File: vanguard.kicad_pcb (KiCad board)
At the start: 4 copper layers, 27.5 x 33.4 mm, 30 parts, among them J1 Conn_01x02, J2 USB_C_Receptacle, J3 Conn_01x04_Pin, J4 Conn_01x02, SW1 Switch_Tactile_CnK, U1 ATtiny3227-M, U2 MCP73831-2-OT, U5 AP63203WU

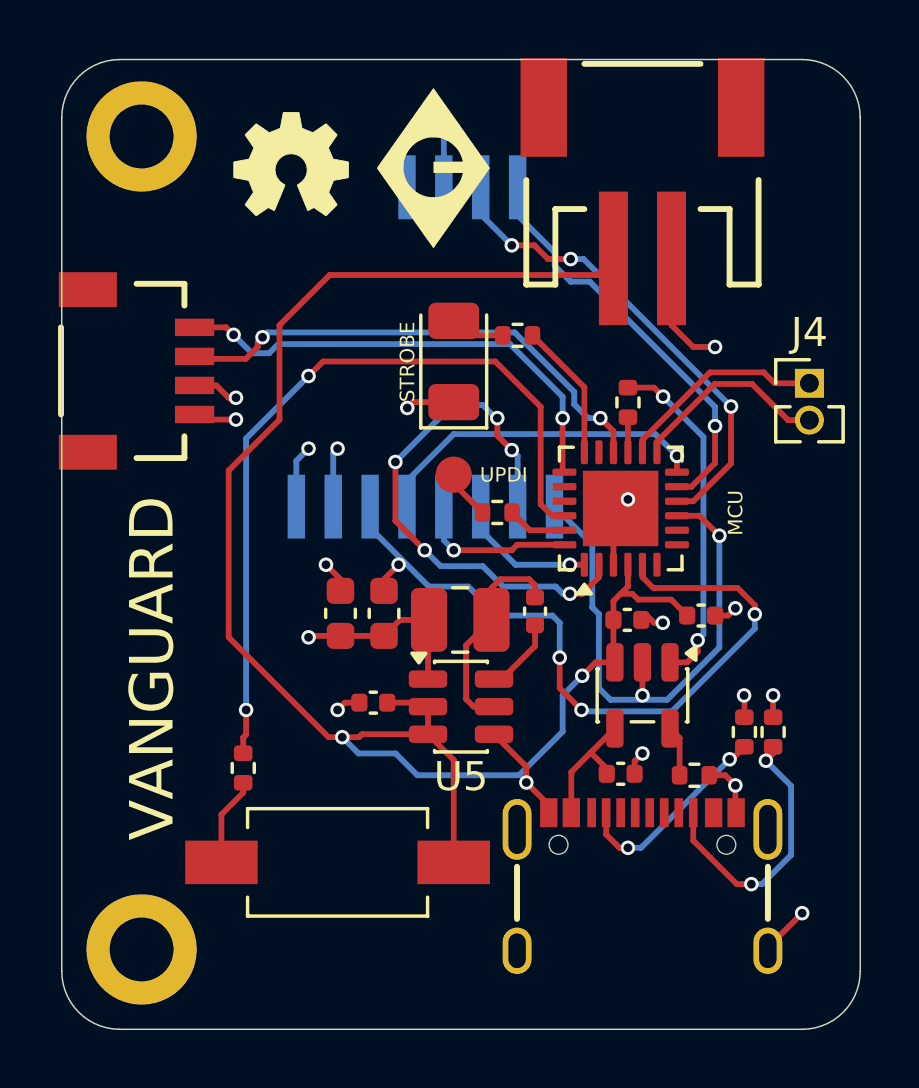
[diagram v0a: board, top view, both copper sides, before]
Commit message: hw check 3
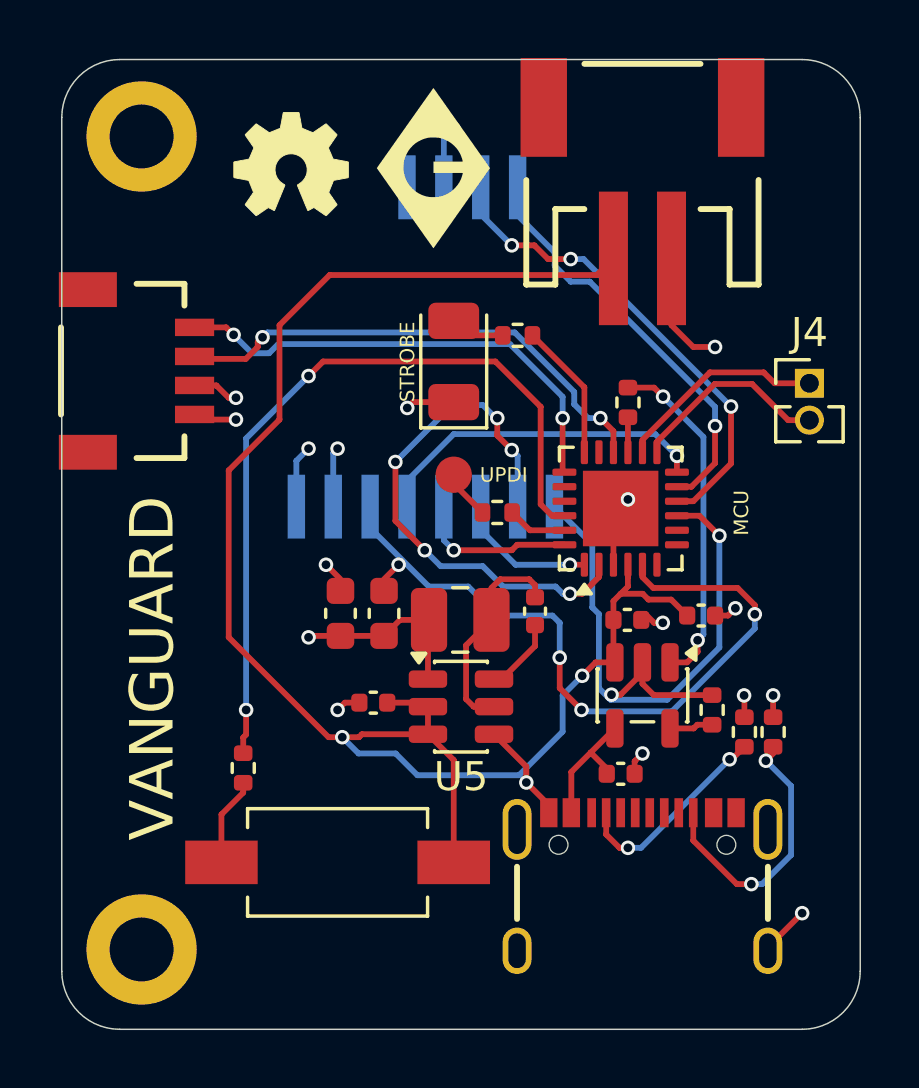
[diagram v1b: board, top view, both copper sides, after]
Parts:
- moved R3 2.33 mm to (144.9, 69.0), turned to -90 degrees
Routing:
- net GND: track 117.3 -> 119.9 mm, vias 18 -> 17
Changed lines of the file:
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@@
 	(footprint "PCM_SparkFun-Resistor:R_0402_1005Metric"
 		(layer "F.Cu")
-		(at 144.29 71.25 180)
+		(at 144.9 69 -90)
 		(descr "Resistor SMD 0402 (1005 Metric), square (rectangular) end terminal, IPC_7351 nominal, (Body size source: IPC-SM-782 page 72, https://www.pcb-3d.com/wordpress/wp-content/uploads/ipc-sm-782a_amendment_1_and_2.pdf), generated with kicad-footprint-generator")
 		(tags "SparkFun resistor")
 		(property "Reference" "R3"
-			(at 0 -1.17 0)
+			(at 0 -1.17 90)
 			(layer "F.Fab")
 			(effects
@@
 		)
 		(property "Value" "2.2k"
-			(at 0 1.17 0)
+			(at 0 1.17 90)
 			(layer "F.Fab")
 			(effects
@@
 		)
 		(property "Datasheet" "https://www.vishay.com/docs/20035/dcrcwe3.pdf"
-			(at 0 0 180)
+			(at 0 0 270)
 			(unlocked yes)
 			(layer "F.Fab")
@@
 		)
 		(property "Description" "Resistor"
-			(at 0 0 180)
+			(at 0 0 270)
 			(unlocked yes)
 			(layer "F.Fab")
@@
 		)
 		(property "PROD_ID" "RES-25566"
-			(at 0 0 180)
+			(at 0 0 270)
 			(unlocked yes)
 			(layer "F.Fab")
@@
 		)
 		(fp_line
-			(start 0.93 0.47)
-			(end -0.93 0.47)
+			(start -0.93 0.47)
+			(end -0.93 -0.47)
 			(stroke
 				(width 0.05)
@@
 		)
 		(fp_line
-			(start 0.93 -0.47)
-			(end 0.93 0.47)
+			(start 0.93 0.47)
+			(end -0.93 0.47)
 			(stroke
 				(width 0.05)
@@
 		)
 		(fp_line
-			(start -0.93 0.47)
-			(end -0.93 -0.47)
+			(start -0.93 -0.47)
+			(end 0.93 -0.47)
 			(stroke
 				(width 0.05)
@@
 		)
 		(fp_line
-			(start -0.93 -0.47)
-			(end 0.93 -0.47)
+			(start 0.93 -0.47)
+			(end 0.93 0.47)
 			(stroke
 				(width 0.05)
@@
 		)
 		(fp_line
-			(start 0.525 0.27)
-			(end -0.525 0.27)
+			(start -0.525 0.27)
+			(end -0.525 -0.27)
 			(stroke
 				(width 0.1)
@@
 		)
 		(fp_line
-			(start 0.525 -0.27)
-			(end 0.525 0.27)
+			(start 0.525 0.27)
+			(end -0.525 0.27)
 			(stroke
 				(width 0.1)
@@
 		)
 		(fp_line
-			(start -0.525 0.27)
-			(end -0.525 -0.27)
+			(start -0.525 -0.27)
+			(end 0.525 -0.27)
 			(stroke
 				(width 0.1)
@@
 		)
 		(fp_line
-			(start -0.525 -0.27)
-			(end 0.525 -0.27)
+			(start 0.525 -0.27)
+			(end 0.525 0.27)
 			(stroke
 				(width 0.1)
@@
 		)
 		(pad "1" smd roundrect
-			(at -0.51 0 180)
+			(at -0.51 0 270)
 			(size 0.54 0.64)
 			(layers "F.Cu" "F.Mask" "F.Paste")
@@
 		)
 		(pad "2" smd roundrect
-			(at 0.51 0 180)
+			(at 0.51 0 270)
 			(size 0.54 0.64)
 			(layers "F.Cu" "F.Mask" "F.Paste")
@@
 	)
 	(gr_text "MCU"
-		(at 146 63 90)
+		(at 146.2 63 90)
 		(layer "F.SilkS")
 		(effects
@@
 	)
 	(segment
-		(start 141.5 64)
-		(end 141.5 62.3125)
+		(start 142.89 68.49)
+		(end 144.9 68.49)
 		(width 0.2)
 		(layer "F.Cu")
@@
 	)
 	(segment
-		(start 145.35 71.25)
-		(end 144.8 71.25)
+		(start 141.5 64)
+		(end 141.5 62.3125)
 		(width 0.2)
 		(layer "F.Cu")
@@
 	)
 	(segment
+		(start 141.747059 68.475)
+		(end 142.5 67.722059)
+		(width 0.2)
+		(layer "F.Cu")
+		(net "GND")
+	)
+	(segment
 		(start 145.45 65.75)
 		(end 145.7 65.5)
@@
 	)
 	(segment
-		(start 143.2 66)
-		(end 142.9 66)
+		(start 142.5 67.3625)
+		(end 142.5 68.1)
 		(width 0.2)
 		(layer "F.Cu")
@@
 	)
 	(segment
-		(start 139.275 72.54)
-		(end 139.275 72.275)
+		(start 143.2 66)
+		(end 142.9 66)
 		(width 0.2)
 		(layer "F.Cu")
@@
 	)
 	(segment
-		(start 145.7 71.6)
-		(end 145.35 71.25)
+		(start 139.275 72.54)
+		(end 139.275 72.275)
 		(width 0.2)
 		(layer "F.Cu")
@@
 	)
 	(segment
-		(start 145.7 71.6)
-		(end 145.7 72.25)
-		(width 0.2)
-		(layer "F.Cu")
-		(net "GND")
-	)
-	(segment
 		(start 145 65.75)
 		(end 145.45 65.75)
@@
 	)
 	(segment
-		(start 142.5 67.3625)
-		(end 142.5 68.5)
-		(width 0.2)
-		(layer "F.Cu")
-		(net "GND")
-	)
-	(segment
 		(start 138.5 70.95)
 		(end 138.5 71.5)
@@
 	)
 	(segment
+		(start 142.5 68.1)
+		(end 142.89 68.49)
+		(width 0.2)
+		(layer "F.Cu")
+		(net "GND")
+	)
+	(segment
 		(start 144.25 56.5)
 		(end 145 56.5)
@@
 	)
 	(segment
+		(start 141.433266 68.475)
+		(end 141.747059 68.475)
+		(width 0.2)
+		(layer "F.Cu")
+		(net "GND")
+	)
+	(segment
 		(start 146.818 77.295)
 		(end 146.818 77.182)
@@
 	)
 	(segment
+		(start 142.5 67.722059)
+		(end 142.5 67.3625)
+		(width 0.2)
+		(layer "F.Cu")
+		(net "GND")
+	)
+	(segment
 		(start 146.01 69.25)
 		(end 146.01 68.51)
@@
 	)
 	(via blind
-		(at 142.5 68.5)
-		(size 0.5)
-		(drill 0.3)
-		(layers "F.Cu" "In1.Cu")
-		(net "GND")
-	)
-	(via blind
 		(at 147 68.5)
 		(size 0.5)
@@
 	)
 	(via blind
-		(at 138.5 71.5)
+		(at 141.433266 68.475)
 		(size 0.5)
 		(drill 0.3)
@@
 	)
 	(via blind
-		(at 145.7 71.6)
+		(at 138.5 71.5)
 		(size 0.5)
 		(drill 0.3)
@@
 	)
 	(segment
+		(start 141.433266 68.475)
+		(end 142.9 67.008266)
+		(width 0.2)
+		(layer "In1.Cu")
+		(net "GND")
+	)
+	(segment
 		(start 142.5 70.5)
 		(end 143.25 71.25)
@@
 	)
 	(segment
-		(start 142.9 68.1)
+		(start 142.9 67.008266)
 		(end 142.9 66.3)
 		(width 0.2)
@@
 	)
 	(segment
-		(start 142.5 68.5)
-		(end 142.9 68.1)
-		(width 0.2)
-		(layer "In1.Cu")
-		(net "GND")
-	)
-	(segment
 		(start 131.6 64)
 		(end 133 64)
@@
 	)
 	(segment
-		(start 140.425 67.825)
-		(end 140.8875 67.3625)
+		(start 143.49 65.2)
+		(end 142.707428 65.2)
 		(width 0.2)
 		(layer "F.Cu")
@@
 	)
 	(segment
-		(start 144.04 65.75)
-		(end 143.49 65.2)
+		(start 140.425 67.825)
+		(end 140.8875 67.3625)
 		(width 0.2)
 		(layer "F.Cu")
@@
 	)
 	(segment
+		(start 144.04 65.75)
+		(end 143.49 65.2)
+		(width 0.2)
+		(layer "F.Cu")
+		(net "VBATT")
+	)
+	(segment
 		(start 140.927818 54.022182)
 		(end 141.5 53.45)
@@
 	)
 	(segment
+		(start 142.507429 65)
+		(end 141.75 65)
+		(width 0.2)
+		(layer "F.Cu")
+		(net "VBATT")
+	)
+	(segment
 		(start 142 64.75)
 		(end 141.75 65)
@@
 	)
 	(segment
-		(start 143.49 65.2)
-		(end 142.35 65.2)
-		(width 0.2)
-		(layer "F.Cu")
-		(net "VBATT")
-	)
-	(segment
-		(start 142.35 65.2)
-		(end 142.15 65)
-		(width 0.2)
-		(layer "F.Cu")
-		(net "VBATT")
-	)
-	(segment
-		(start 142.15 65)
-		(end 141.75 65)
-		(width 0.2)
-		(layer "F.Cu")
-		(net "VBATT")
-	)
-	(segment
 		(start 132.161091 69.938909)
 		(end 131.688909 69.938909)
@@
 	)
 	(segment
+		(start 142.707428 65.2)
+		(end 142.507429 65)
+		(width 0.2)
+		(layer "F.Cu")
+		(net "VBATT")
+	)
+	(segment
 		(start 134.975 68.75)
 		(end 135.1125 68.8875)
@@
 	)
 	(segment
-		(start 143.78 69.9675)
-		(end 143.78 71.25)
+		(start 144.2625 69.6375)
+		(end 143.45 69.6375)
+		(width 0.2)
+		(layer "F.Cu")
+		(net "Net-(U2-PROG)")
+	)
+	(segment
+		(start 144.9 69.51)
+		(end 144.39 69.51)
 		(width 0.2)
 		(layer "F.Cu")
@@
 	)
 	(segment
-		(start 143.45 69.6375)
-		(end 143.78 69.9675)
+		(start 144.39 69.51)
+		(end 144.2625 69.6375)
 		(width 0.2)
 		(layer "F.Cu")
